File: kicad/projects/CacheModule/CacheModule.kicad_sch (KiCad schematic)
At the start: 20 parts, among them U1 CY7C1041D, U2 CY7C1041D, U3 CY7C1041D, U4 CY7C1041D, U5 CY7C1041D, U6 24LC00

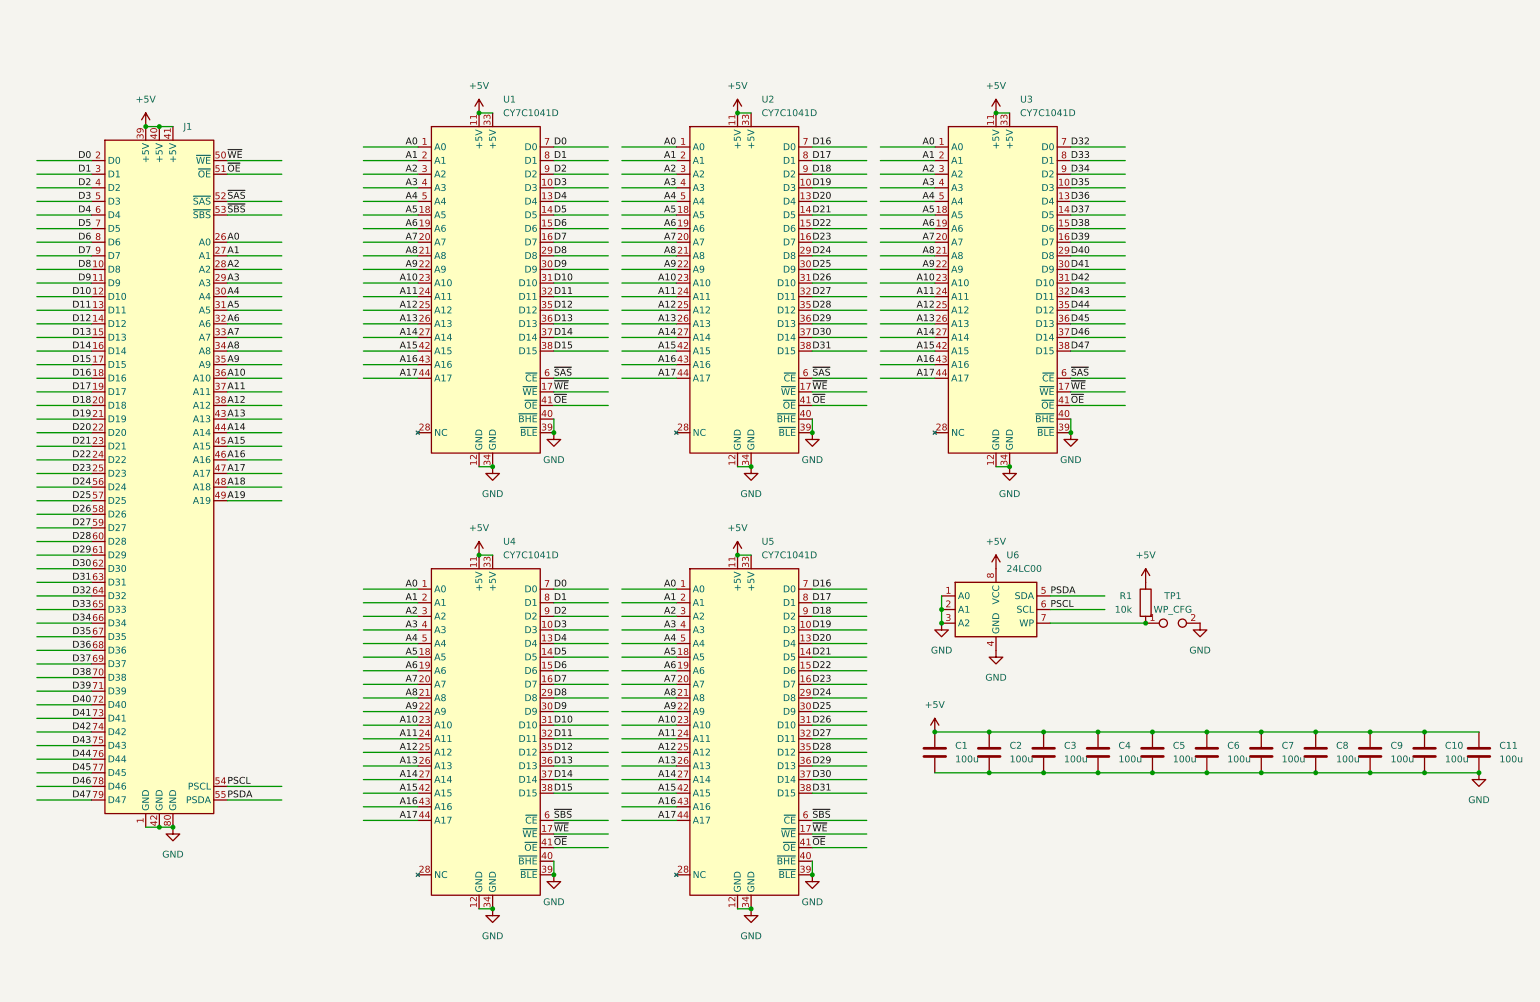
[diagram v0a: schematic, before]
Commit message: Some Updates
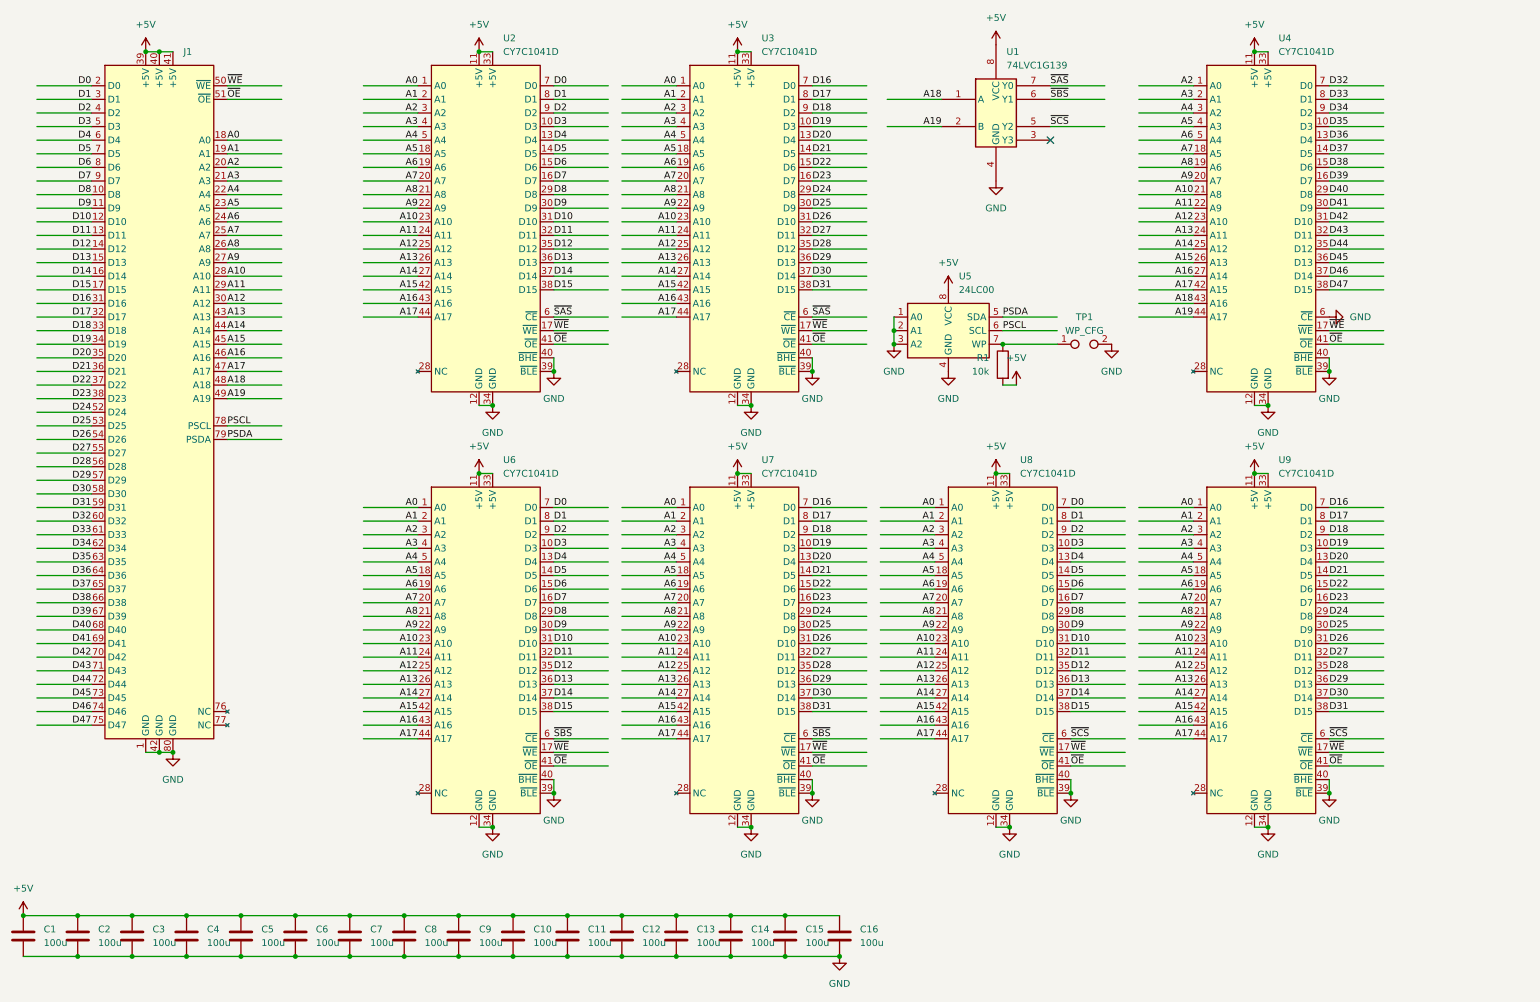
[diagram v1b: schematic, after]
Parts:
- added C12, C13, C14, C15, C16: 100u, Capacitor_SMD:C_0603_1608Metric_Pad1.08x0.95mm_HandSolder, symbol Device:C
- added U1: 74LVC1G139, Package_SO:SSOP-8_3.9x5.05mm_P1.27mm, symbol 74xGxx:74LVC1G139
- added U8, U9: CY7C1041D, Package_SO:TSOP-II-44_10.16x18.41mm_P0.8mm, symbol m68k-hbc-ic:CY7C1041D
- J1: footprint m68k-hbc-conn:SIMM80_Cache_CardEdge -> m68k-hbc-conn:SIMM80_CardEdge; symbol m68k-hbc-conn:SIMM80_Cache_CardEdge -> m68k-hbc-conn:SIMM80_Cache
- TP1: footprint Connector_PinHeader_1.27mm:PinHeader_1x02_P1.27mm_Vertical -> Resistor_SMD:R_0402_1005Metric
- renumbered U1 to U2, U2 to U3, U3 to U4, U6 to U5, U4 to U6, U5 to U7
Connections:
- net +5V: now also R1.2, C12.1, C13.1, C14.1, C15.1, C16.1, U1.8 (VCC), U8.11 (+5V), U8.33 (+5V), U9.11 (+5V), U9.33 (+5V); no longer R1.1
- net A0: now also J1.18 (A0), U8.1 (A0), U9.1 (A0); no longer J1.26 (A0), U4.1 (A0)
- net A1: now also J1.19 (A1), U8.2 (A1), U9.2 (A1); no longer J1.27 (A1), U4.2 (A1)
- net A10: now also J1.28 (A10), U4.21 (A8), U8.23 (A10), U9.23 (A10); no longer J1.36 (A10), U4.23 (A10)
- net A11: now also J1.29 (A11), U4.22 (A9), U8.24 (A11), U9.24 (A11); no longer J1.37 (A11), U4.24 (A11)
- net A12: now also J1.30 (A12), U4.23 (A10), U8.25 (A12), U9.25 (A12); no longer J1.38 (A12), U4.25 (A12)
- net A13: now also U4.24 (A11), U8.26 (A13), U9.26 (A13); no longer U4.26 (A13)
- net A14: now also U4.25 (A12), U8.27 (A14), U9.27 (A14); no longer U4.27 (A14)
- net A15: now also U4.26 (A13), U8.42 (A15), U9.42 (A15); no longer U4.42 (A15)
- net A16: now also U4.27 (A14), U8.43 (A16), U9.43 (A16); no longer U4.43 (A16)
- net A17: now also U4.42 (A15), U8.44 (A17), U9.44 (A17); no longer U4.44 (A17)
- net A18: now also U4.43 (A16), U1.1 (A)
- net A19: now also U4.44 (A17), U1.2 (B)
- net A2: now also J1.20 (A2), U4.1 (A0), U8.3 (A2), U9.3 (A2); no longer J1.28 (A2), U4.3 (A2)
- net A3: now also J1.21 (A3), U4.2 (A1), U8.4 (A3), U9.4 (A3); no longer J1.29 (A3), U4.4 (A3)
- net A4: now also J1.22 (A4), U4.3 (A2), U8.5 (A4), U9.5 (A4); no longer J1.30 (A4), U4.5 (A4)
- net A5: now also J1.23 (A5), U4.4 (A3), U8.18 (A5), U9.18 (A5); no longer J1.31 (A5), U4.18 (A5)
- net A6: now also J1.24 (A6), U4.5 (A4), U8.19 (A6), U9.19 (A6); no longer J1.32 (A6), U4.19 (A6)
- net A7: now also J1.25 (A7), U4.18 (A5), U8.20 (A7), U9.20 (A7); no longer J1.33 (A7), U4.20 (A7)
- net A8: now also J1.26 (A8), U4.19 (A6), U8.21 (A8), U9.21 (A8); no longer J1.34 (A8), U4.21 (A8)
- net A9: now also J1.27 (A9), U4.20 (A7), U8.22 (A9), U9.22 (A9); no longer J1.35 (A9), U4.22 (A9)
- net D0: now also U8.7 (D0)
- net D1: now also U8.8 (D1)
- net D10: now also U8.31 (D10)
- net D11: now also U8.32 (D11)
- net D12: now also U8.35 (D12)
- net D13: now also U8.36 (D13)
- net D14: now also U8.37 (D14)
- net D15: now also U8.38 (D15)
- net D16: now also J1.31 (D16), U9.7 (D0); no longer J1.18 (D16)
- net D17: now also J1.32 (D17), U9.8 (D1); no longer J1.19 (D17)
- net D18: now also J1.33 (D18), U9.9 (D2); no longer J1.20 (D18)
- net D19: now also J1.34 (D19), U9.10 (D3); no longer J1.21 (D19)
- net D2: now also U8.9 (D2)
- net D20: now also J1.35 (D20), U9.13 (D4); no longer J1.22 (D20)
- net D21: now also J1.36 (D21), U9.14 (D5); no longer J1.23 (D21)
- net D22: now also J1.37 (D22), U9.15 (D6); no longer J1.24 (D22)
- net D23: now also J1.38 (D23), U9.16 (D7); no longer J1.25 (D23)
- net D24: now also J1.52 (D24), U9.29 (D8); no longer J1.56 (D24)
- net D25: now also J1.53 (D25), U9.30 (D9); no longer J1.57 (D25)
- net D26: now also J1.54 (D26), U9.31 (D10); no longer J1.58 (D26)
- net D27: now also J1.55 (D27), U9.32 (D11); no longer J1.59 (D27)
- net D28: now also J1.56 (D28), U9.35 (D12); no longer J1.60 (D28)
- net D29: now also J1.57 (D29), U9.36 (D13); no longer J1.61 (D29)
- net D3: now also U8.10 (D3)
- net D30: now also J1.58 (D30), U9.37 (D14); no longer J1.62 (D30)
- net D31: now also J1.59 (D31), U9.38 (D15); no longer J1.63 (D31)
- net D32: now also J1.60 (D32); no longer J1.64 (D32)
- net D33: now also J1.61 (D33); no longer J1.65 (D33)
- net D34: now also J1.62 (D34); no longer J1.66 (D34)
- net D35: now also J1.63 (D35); no longer J1.67 (D35)
- net D36: now also J1.64 (D36); no longer J1.68 (D36)
- net D37: now also J1.65 (D37); no longer J1.69 (D37)
- net D38: now also J1.66 (D38); no longer J1.70 (D38)
- net D39: now also J1.67 (D39); no longer J1.71 (D39)
- net D4: now also U8.13 (D4)
- net D40: now also J1.68 (D40); no longer J1.72 (D40)
- net D41: now also J1.69 (D41); no longer J1.73 (D41)
- net D42: now also J1.70 (D42); no longer J1.74 (D42)
- net D43: now also J1.71 (D43); no longer J1.75 (D43)
- net D44: now also J1.72 (D44); no longer J1.76 (D44)
- net D45: now also J1.73 (D45); no longer J1.77 (D45)
- net D46: now also J1.74 (D46); no longer J1.78 (D46)
- net D47: now also J1.75 (D47); no longer J1.79 (D47)
- net D5: now also U8.14 (D5)
- net D6: now also U8.15 (D6)
- net D7: now also U8.16 (D7)
- net D8: now also U8.29 (D8)
- net D9: now also U8.30 (D9)
- net GND: now also U4.6 (~{CE}), C12.2, C13.2, C14.2, C15.2, C16.2, U1.4 (GND), U8.12 (GND), U8.34 (GND), U8.39 (~{BLE}), U8.40 (~{BHE}), U9.12 (GND), U9.34 (GND), U9.39 (~{BLE}), U9.40 (~{BHE})
- net PSCL: now also J1.78 (PSCL); no longer J1.54 (PSCL)
- net PSDA: now also J1.79 (PSDA); no longer J1.55 (PSDA)
- net ~{OE}: now also U8.41 (~{OE}), U9.41 (~{OE})
- net ~{SAS}: now also U1.7 (Y0); no longer J1.52 (~{SAS}), U4.6 (~{CE})
- net ~{SBS}: now also U1.6 (Y1); no longer J1.53 (~{SBS})
- net ~{WE}: now also U8.17 (~{WE}), U9.17 (~{WE})
- net at TP1.1, U5.7 (WP): now also R1.1; no longer R1.2
- new net ~{SCS}: U1.5 (Y2), U8.6 (~{CE}), U9.6 (~{CE})
- no-connect marks 0 -> 1
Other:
- moved on the sheet: C1, C2, C3, C4, C5, C6, C7, C8, TP1, U2, U3, U4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
